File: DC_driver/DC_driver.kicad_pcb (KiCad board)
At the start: 2 copper layers, 56.6 x 73.9 mm, 38 parts, among them J1 CONN_01X10, J2 CONN_01X10, J3 CONN_01X10, J4 CONN_01X10, P1 CONN_01X02, P2 CONN_01X02, U1 MC34063A, U2 NTD3055L104-D, U3 NTD3055L104-D, U4 NTD3055L104-D, U5 NTD3055L104-D

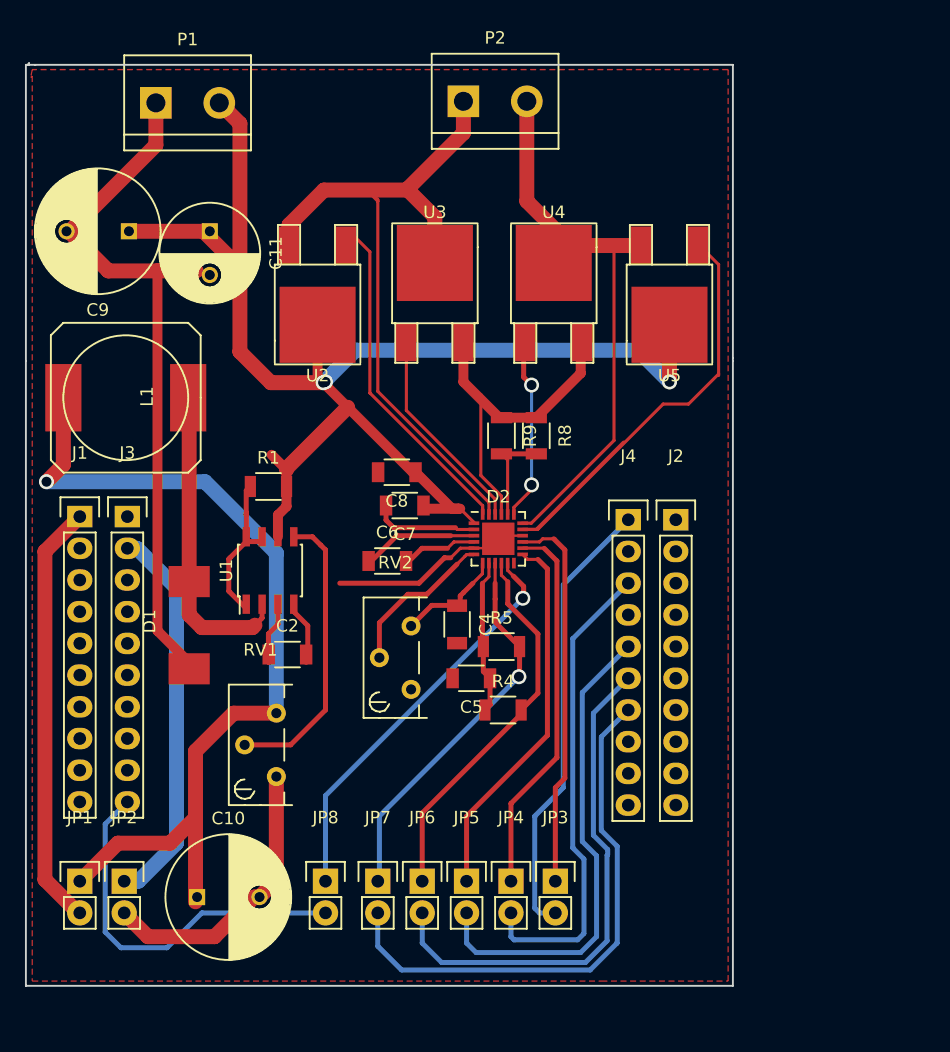
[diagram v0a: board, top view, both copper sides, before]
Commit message: main changes
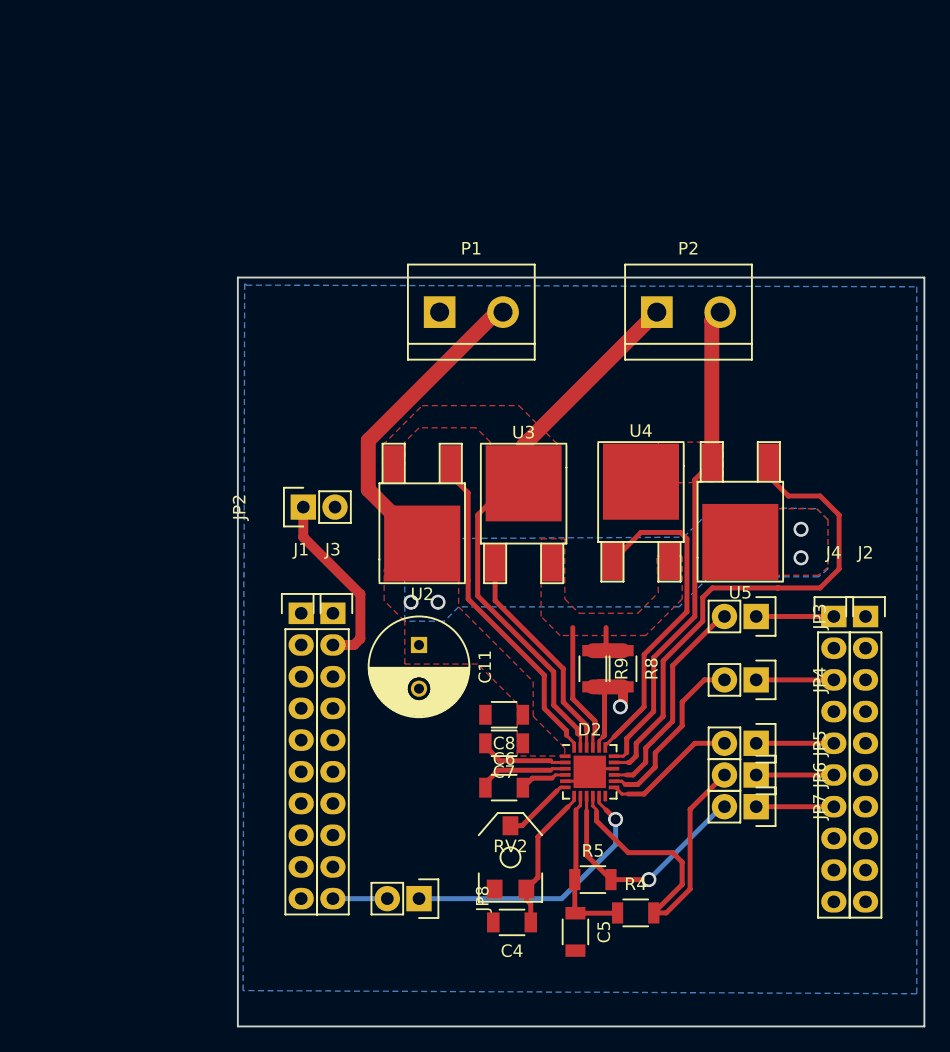
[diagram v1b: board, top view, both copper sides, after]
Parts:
- removed C10, C9: 470 uF, Capacitors_ThroughHole:C_Radial_D10_L21_P5
- removed C2: C, Capacitors_SMD:C_1206
- removed D1: D_Schottky, Diodes_SMD:9.40x3.30
- removed JP1: JUMPER, Pin_Headers:Pin_Header_Straight_1x02
- removed L1: L_Small, Inductors:SELF-WE-PD-XXL
- removed R1: R, Resistors_SMD:R_1206
- removed RV1: POT, Potentiometers:Potentiometer_Bourns_3296Y_3-8Zoll_Angular_ScrewUp
- removed U1: MC34063A, Housings_SOIC:SOIC-8_3.9x4.9mm_Pitch1.27mm
- RV2: footprint Potentiometers:Potentiometer_Bourns_3296Y_3-8Zoll_Angular_ScrewUp -> SMD_Packages:POT_SMD
- moved C11 37.1 mm to (112.0, 99.4)
- moved JP2 33.2 mm to (102.7, 88.4), turned to 90 degrees
- moved JP7 30.9 mm to (139.0, 112.4), turned to 270 degrees
- moved P1 28.2 mm to (116.2, 72.8)
- moved JP6 28.1 mm to (139.0, 109.9), turned to 270 degrees
- moved JP3 26.6 mm to (139.0, 97.2), turned to 270 degrees
- moved JP5 25.7 mm to (139.0, 107.3), turned to 270 degrees
- moved JP4 25.4 mm to (139.0, 102.2), turned to 270 degrees
- moved C4 24.3 mm to (119.5, 121.7), turned to 180 degrees
- moved P2 22.9 mm to (133.6, 72.8)
- moved C5 22.0 mm to (124.5, 122.4), turned to 270 degrees
- moved C8 21.2 mm to (118.8, 105.0)
- moved C7 20.6 mm to (118.8, 107.3)
- moved C6 20.4 mm to (118.8, 110.9)
- moved R5 20.1 mm to (125.9, 118.2)
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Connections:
- J4 pad 1: /P40 -> /P40A
- J4 pad 3: /P38 -> /P38A
- J4 pad 5: /P36 -> /P36A
- J4 pad 6: /P35 -> /P35A
- J4 pad 7: /P34 -> /P34A
- JP3 pad 1: /P40 -> /P40A
- JP4 pad 1: /P38 -> /P38A
- JP5 pad 1: /P36 -> /P36A
- JP6 pad 1: /P35 -> /P35A
- JP7 pad 1: /P34 -> /P34A
- JP8 pad 1: /A1 -> /A1A
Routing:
- net +3V3: track 106.2 -> 0.00 mm, vias 1 -> 0
- net GND: track 109.2 -> 12.9 mm
- net VM: track 112.3 -> 25.1 mm, vias 3 -> 0
- net /P36: track 69.1 -> 10.7 mm
- net /A1: track 63.4 -> 6.77 mm, vias 1 -> 0
- net /P34: track 75.1 -> 19.1 mm
- net /P38: track 68.7 -> 14.2 mm
- net /P40: track 67.9 -> 17.4 mm
- net /P35: track 71.8 -> 29.3 mm
- net Net-(D1-Pad1): track 24.7 -> 0.00 mm
- net Net-(RV1-Pad2): track 23.4 -> 0.00 mm
- net /A1A: track 0.00 -> 19.2 mm, vias 0 -> 1
- net GNDA: track 31.4 -> 14.8 mm
- net Net-(D2-Pad21): track 29.8 -> 14.7 mm
- net Net-(D2-Pad23): track 59.4 -> 45.4 mm
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- added copper zone on B.Cu, net GND
- added copper zone on F.Cu, net Net-(D2-Pad18)
- added copper zone on F.Cu, net Net-(D2-Pad21)
- added copper zone on F.Cu, net Net-(D2-Pad23)
- added copper zone on B.Cu, net VM
- added copper zone on F.Cu, net VM
- removed copper zone on F.Cu, net GND
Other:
- board size 56.6 x 73.9 mm -> 55 x 60 mm
